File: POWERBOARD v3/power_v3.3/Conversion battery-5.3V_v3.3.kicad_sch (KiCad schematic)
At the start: 11 parts, among them U3 TPS62160DSG

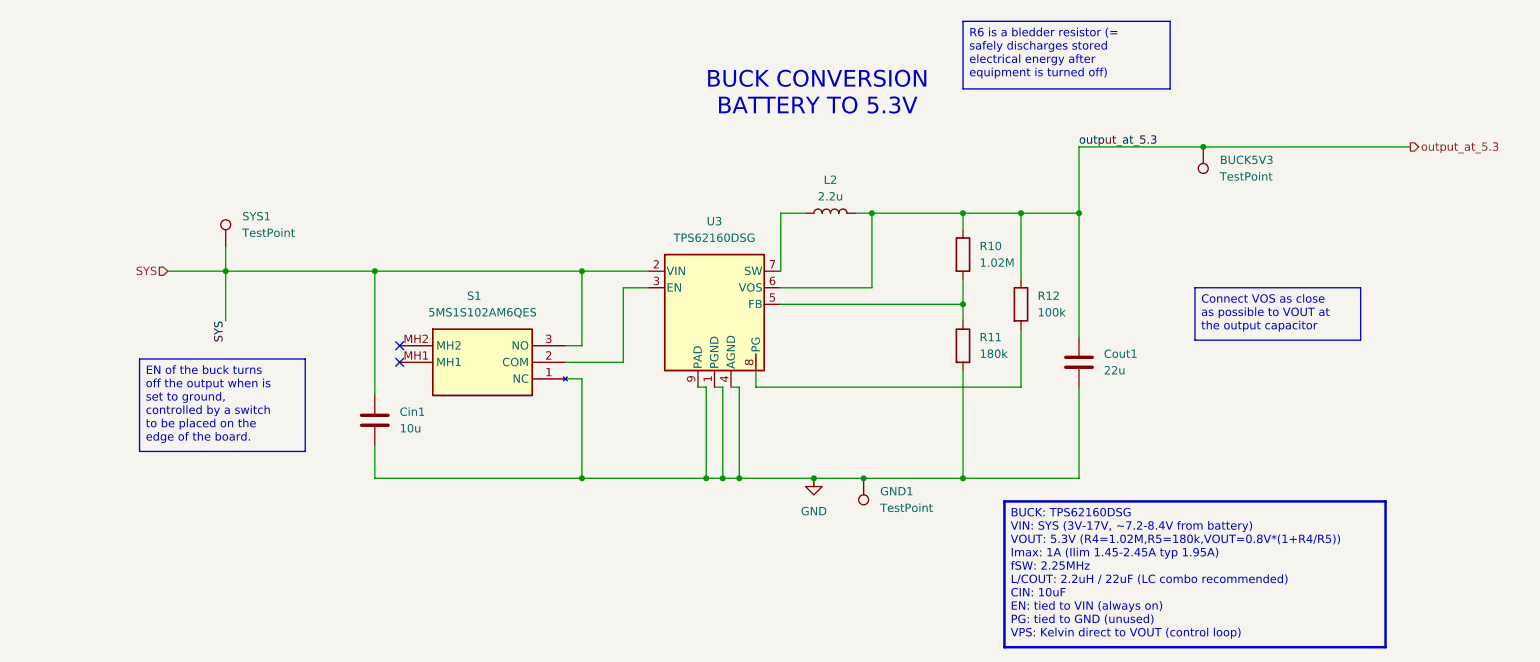
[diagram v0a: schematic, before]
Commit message: (nearly) finished schematic and layout, beginning routing (hooooooly)
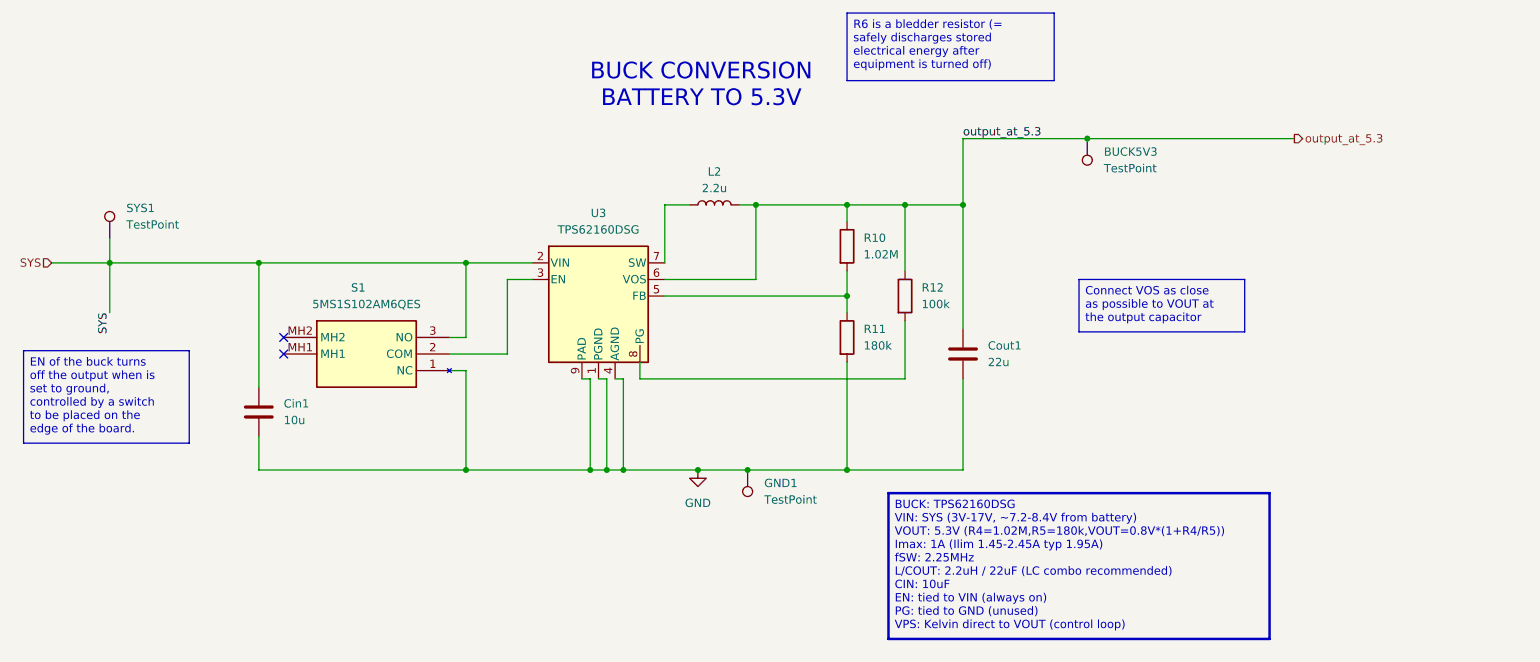
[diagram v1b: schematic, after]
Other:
- moved on the sheet: BUCK5V3, Cin1, Cout1, GND1, L2, R10, R11, R12, S1, SYS1, U3
